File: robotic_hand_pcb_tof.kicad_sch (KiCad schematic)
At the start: 1 part, among them J5 Conn_01x04_Pin

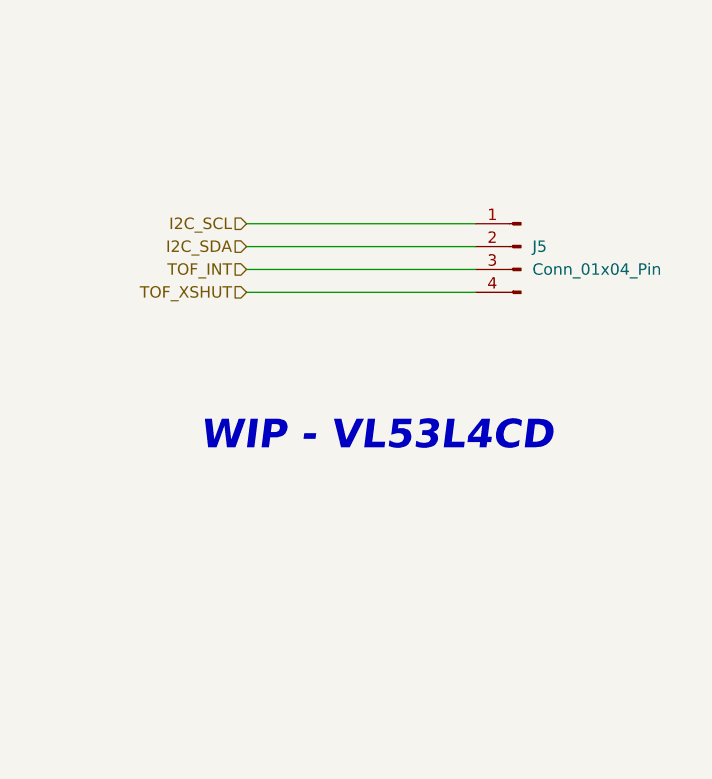
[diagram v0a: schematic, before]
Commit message: Add WIP schematic changes
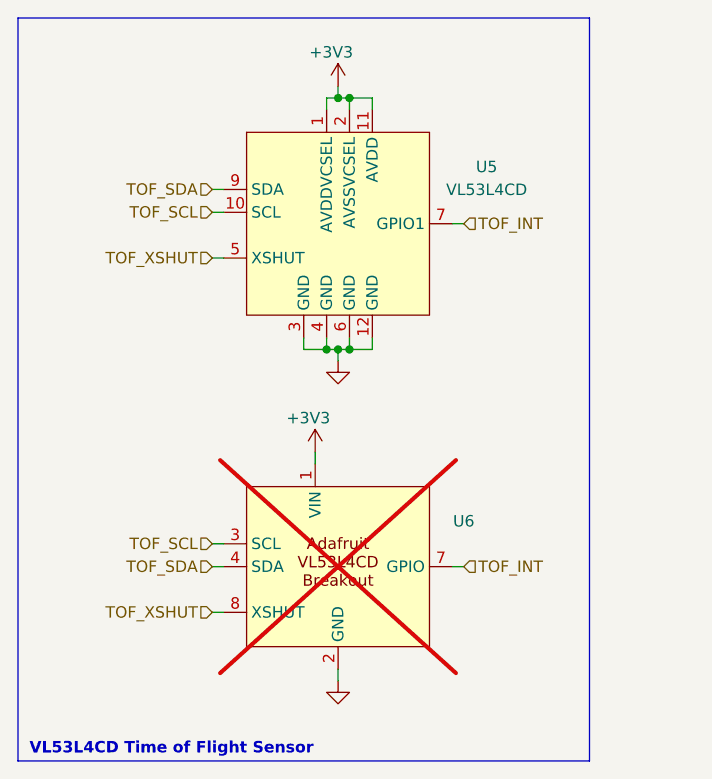
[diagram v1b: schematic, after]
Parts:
- removed J5: Conn_01x04_Pin, symbol Connector:Conn_01x04_Pin
- added U5: VL53L4CD, time_of_flight:vl53l4cd_lga12, symbol time_of_flight:vl53l4cd
- added U6: ~, adafruit:adafruit_5396_vl53l4cd, symbol adafruit:adafruit_5396_vl53l4cd
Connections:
- net TOF_INT: now also U5.7 (GPIO1), U6.7 (GPIO)
- net TOF_XSHUT: now also U5.5 (XSHUT), U6.8 (XSHUT)
- new net +3V3: U5.1 (AVDDVCSEL), U5.11 (AVDD), U5.2 (AVSSVCSEL), U6.1 (VIN)
- new net GND: U5.12 (GND), U5.3 (GND), U5.4 (GND), U5.6 (GND), U6.2 (GND)
- new net TOF_SCL: U5.10 (SCL), U6.3 (SCL)
- new net TOF_SDA: U5.9 (SDA), U6.4 (SDA)
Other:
- note added: "VL53L4CD Time of Flight Sensor"
- note removed: "WIP - VL53L4CD"
